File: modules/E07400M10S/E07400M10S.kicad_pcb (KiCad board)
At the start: 2 copper layers, 25.4 x 28.6 mm, 14 parts, among them J1 Conn_01x08, J2 Conn_01x08, U1 E07-400M10S

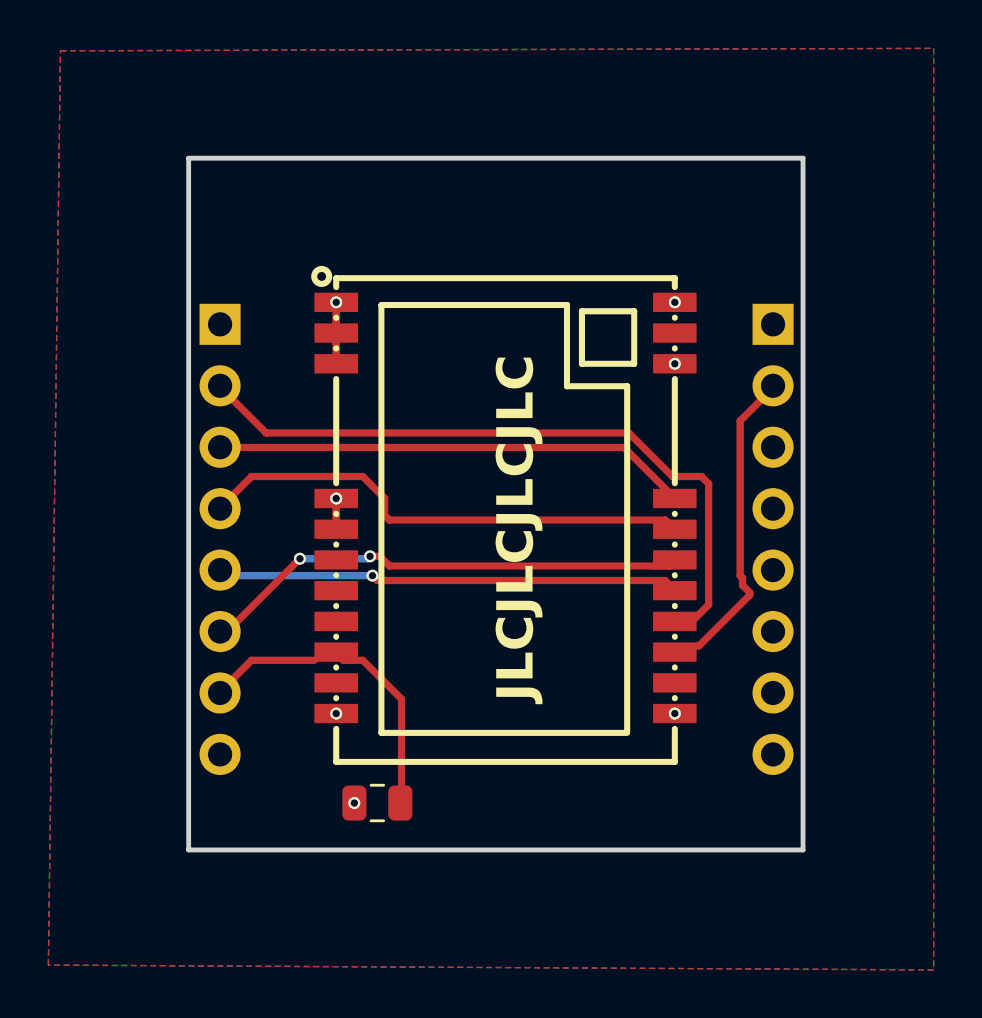
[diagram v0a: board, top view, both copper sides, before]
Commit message: cross check E07400M10S is ready for fabrication
Signed-off-by: Rodney Osodo <socials@rodneyosodo.com>
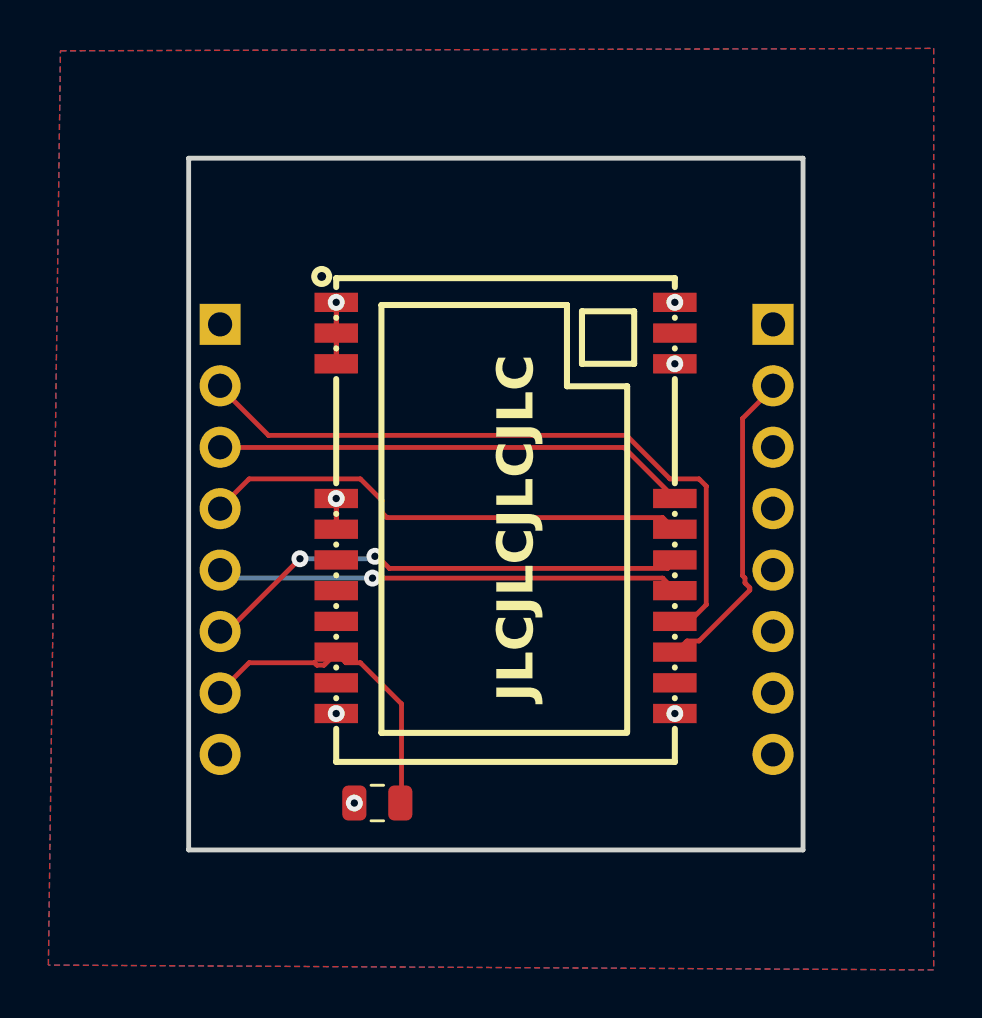
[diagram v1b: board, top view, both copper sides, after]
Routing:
- net +3V3: track 12.3 -> 13.3 mm
